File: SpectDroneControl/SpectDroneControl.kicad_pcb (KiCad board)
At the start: 2 copper layers, 101.7 x 73.7 mm, 165 parts, among them J1 Conn_02x03_Counter_Clockwise, J2-1 Conn_01x04_Male, J2-2 Conn_01x04_Male, J3-1 Conn_01x01_Female, J3-2 Conn_01x01_Female, J3-3 Conn_01x01_Female, J3-4 Conn_01x01_Female, J3-5 Conn_01x01_Female, J3V1 Conn_01x01_Male, J5-1 Conn_01x01_Female, J5-2 Conn_01x01_Female, J5-3 Conn_01x01_Female, J5-4 Conn_01x01_Female, J5-5 Conn_01x01_Female, J5V1 Conn_01x01_Female, Q1 FDN340P, Q2 Q_NPN_EBC, SW1 SW_SPDT, U1 Teensy4.1, U2 LM7805_SOT223, U3 MCP112-450E/TO, U4 NVT2010PW, U5 NVT2010PW, U6 NVT2010PW, U7 TXS0102DCUR

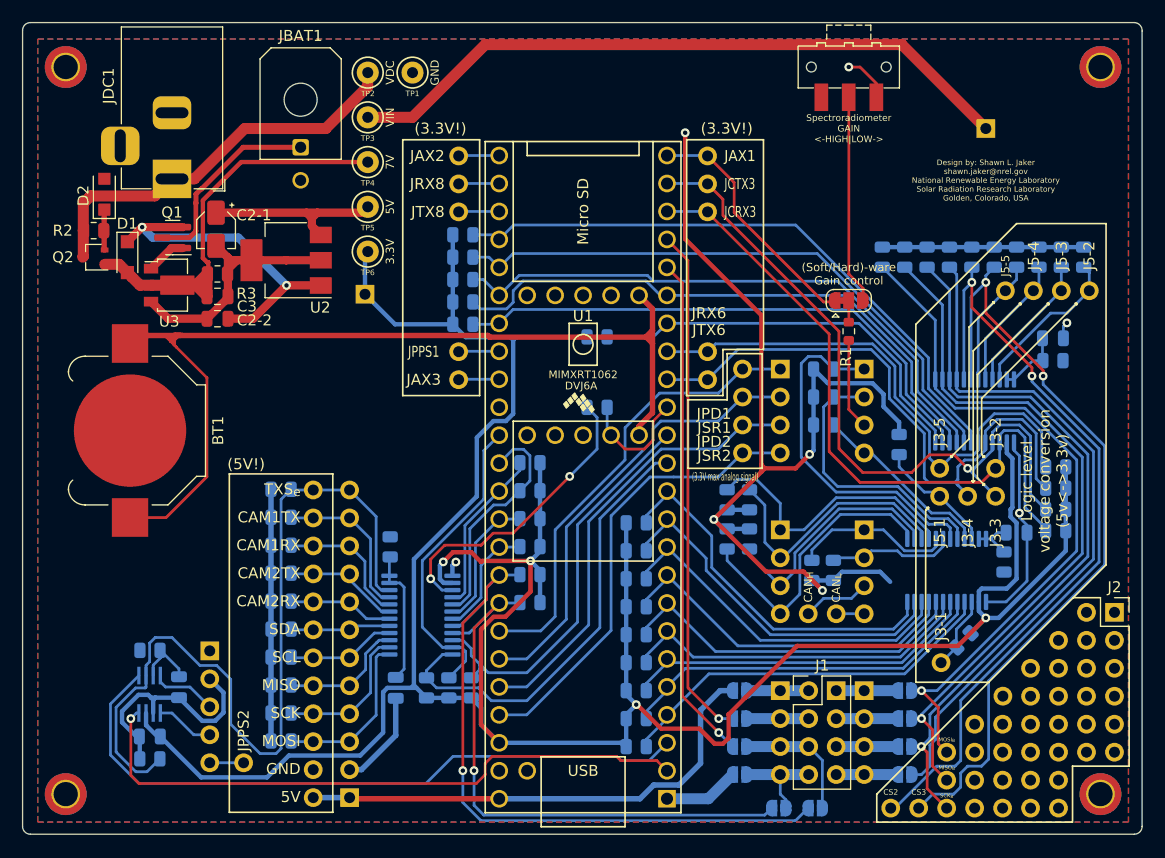
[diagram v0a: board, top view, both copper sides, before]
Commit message: SpectDrone Development
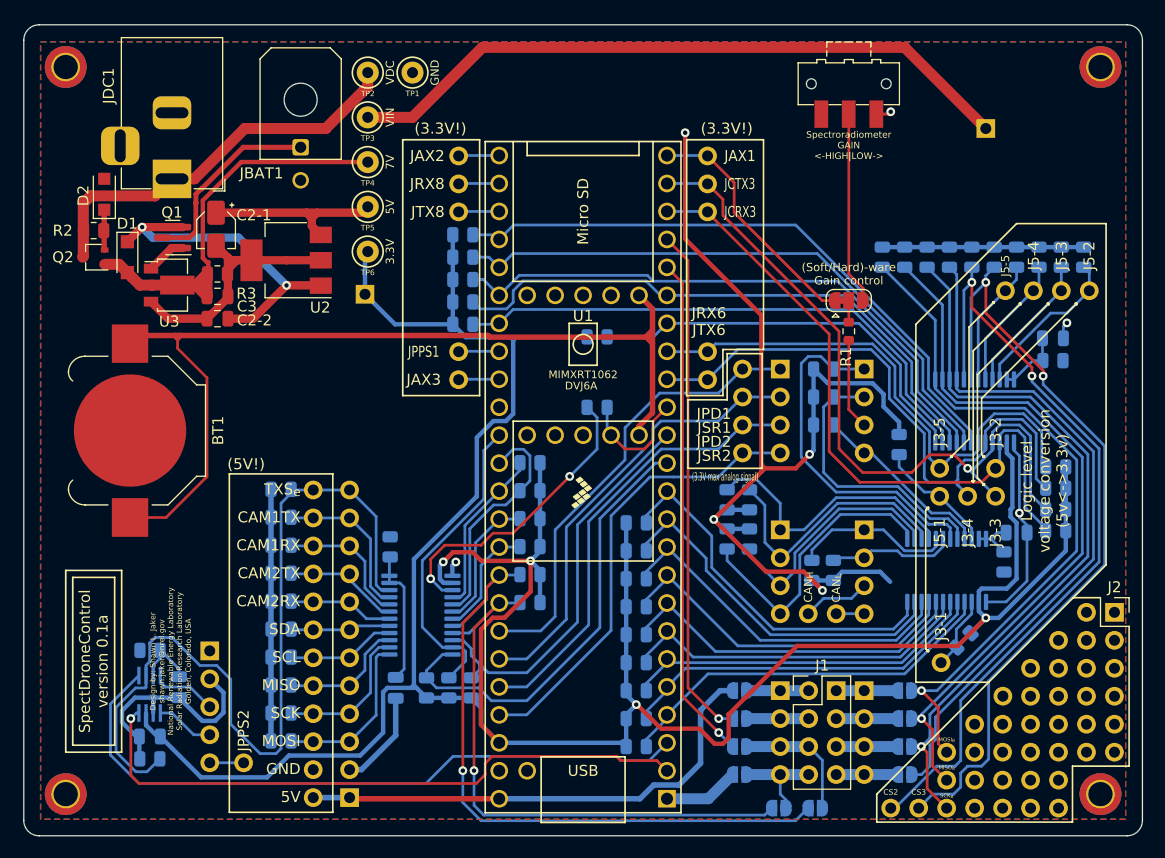
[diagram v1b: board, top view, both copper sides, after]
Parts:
- moved SW1 1.52 mm to (174.9, 68.5)
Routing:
- net /VBat: track 89.3 -> 85.8 mm
- net /5V: track 201.3 -> 198.4 mm
- net Net-(JPAX1-Pad3): track 19.0 -> 17.5 mm
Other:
- board size 101.7 x 73.7 mm -> 101.6 x 73.7 mm
- board text added: "SpectDroneControl version 0.1a"
